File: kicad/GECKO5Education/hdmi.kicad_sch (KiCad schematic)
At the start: 20 parts, among them J2 HDMI_A, U3 PCA9306DQER, U6 LFE5U-85F-6BG381x

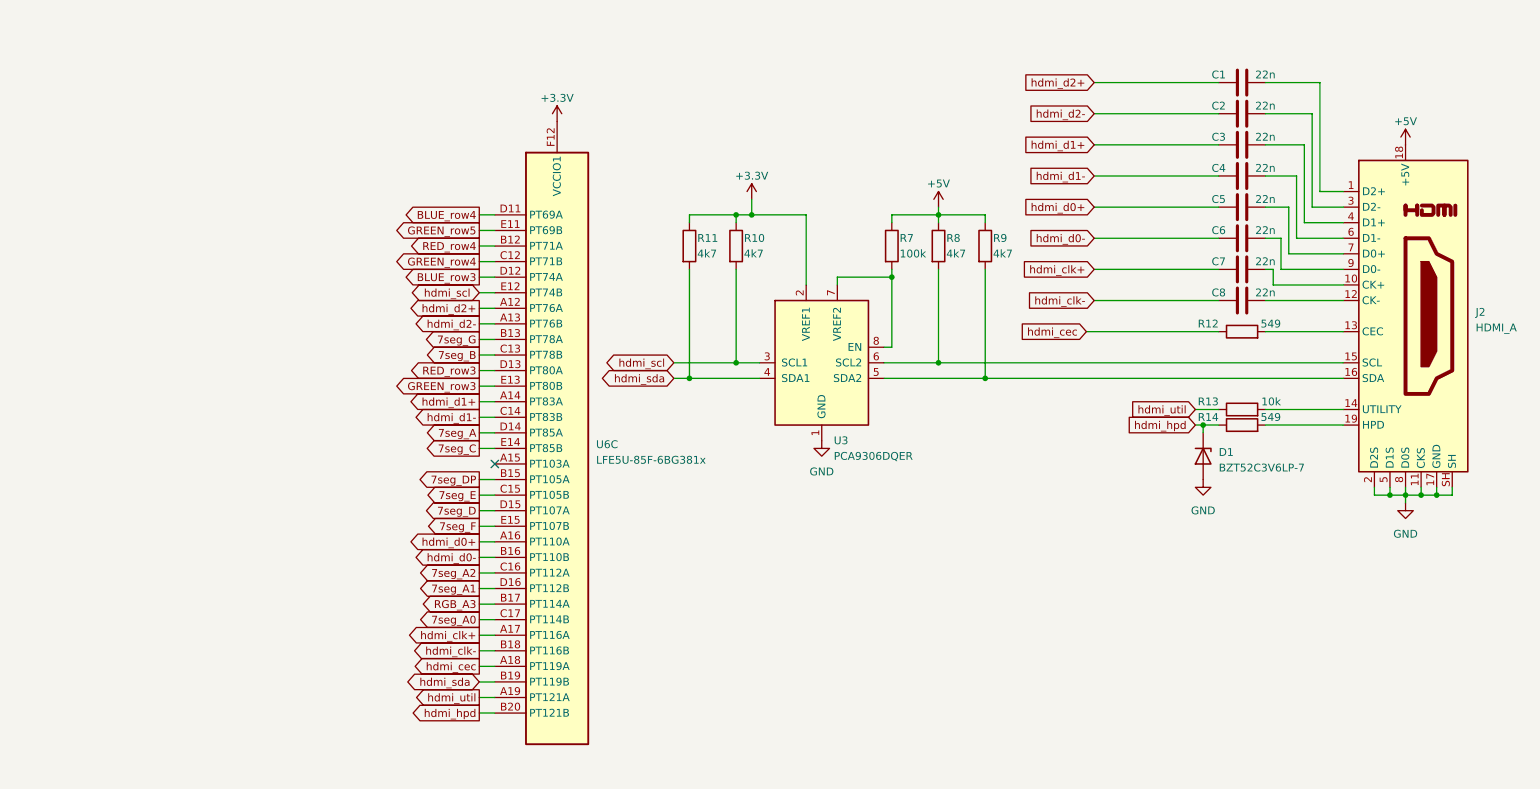
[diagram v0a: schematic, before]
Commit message: Made version V1.5
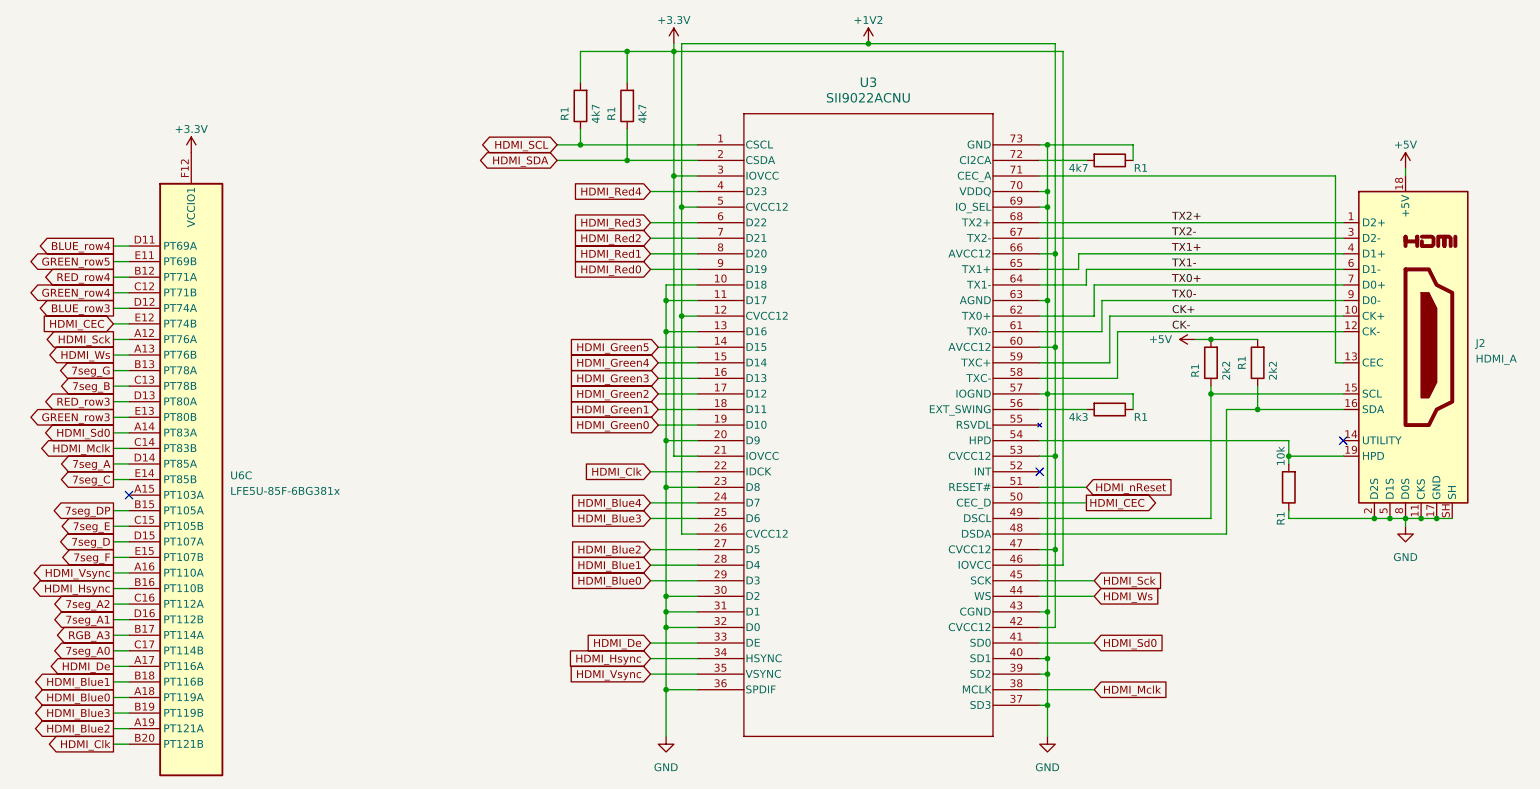
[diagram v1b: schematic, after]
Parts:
- removed C1, C2, C3, C4, C5, C6, C7, C8: 22n, Capacitor_SMD:C_0402_1005Metric, symbol Device:C
- removed D1: BZT52C3V6LP-7, Diode_SMD:D_0402_1005Metric, symbol Device:D_Zener
- removed R10, R11, R8, R9: 4k7, Resistor_SMD:R_0402_1005Metric, symbol Device:R
- removed R12, R14: 549, Resistor_SMD:R_0402_1005Metric, symbol Device:R
- removed R13: 10k, Resistor_SMD:R_0402_1005Metric, symbol Device:R
- removed R7: 100k, Resistor_SMD:R_0402_1005Metric, symbol Device:R
- removed U3: PCA9306DQER, Package_SON:X2SON-8_1.4x1mm_P0.35mm, symbol Interface:PCA9306
- added R1 (x3): 4k7, Resistor_SMD:R_0402_1005Metric, symbol Device:R
- added R1: 10k, Resistor_SMD:R_0402_1005Metric, symbol Device:R
- added R1: 4k3, Resistor_SMD:R_0402_1005Metric, symbol Device:R
- added R1 (x2): 2k2, Resistor_SMD:R_0402_1005Metric, symbol Device:R
- added U3: SII9022ACNU, gecko4education:QFN72_10X10_LAT-M, symbol gecko5education:SII9022ACNU
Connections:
- net +3.3V: now also R1.2, R1.2, U3.21 (IOVCC), U3.3 (IOVCC), U3.46 (IOVCC)
- net +5V: now also R1.2, R1.2
- net GND: now also R1.1, R1.1, R1.1, U3.10 (D18), U3.11 (D17), U3.13 (D16), U3.20 (D9), U3.23 (D8), U3.30 (D2), U3.31 (D1), U3.32 (D0), U3.36 (SPDIF), U3.37 (SD3), U3.39 (SD2), U3.40 (SD1), U3.43 (CGND), U3.57 (IOGND), U3.63 (AGND), U3.69 (IO_SEL), U3.70 (VDDQ), U3.73 (GND)
- net at J2.13 (CEC): now also U3.71 (CEC_A)
- net CK+: now reaches J2.10 (CK+)
- net CK+: now also U3.59 (TXC+)
- net CK-: now reaches J2.12 (CK-)
- net CK-: now also U3.58 (TXC-)
- net TX2+: now reaches J2.1 (D2+)
- net TX2+: now also U3.68 (TX2+)
- net TX1-: now reaches J2.6 (D1-)
- net TX1-: now also U3.64 (TX1-)
- net TX0+: now reaches J2.7 (D0+)
- net TX0+: now also U3.62 (TX0+)
- net TX1+: now reaches J2.4 (D1+)
- net TX1+: now also U3.65 (TX1+)
- net at J2.15 (SCL): now also R1.1, U3.49 (DSCL)
- net at J2.16 (SDA): now also R1.1, U3.48 (DSDA)
- net at J2.19 (HPD): now also R1.2, U3.54 (HPD)
- net TX2-: now reaches J2.3 (D2-)
- net TX2-: now also U3.67 (TX2-)
- net TX0-: now reaches J2.9 (D0-)
- net TX0-: now also U3.61 (TX0-)
- net hdmi_cec renamed HDMI_Blue0
- net HDMI_Blue0: now also U3.29 (D3)
- net hdmi_clk+ renamed HDMI_De
- net HDMI_De: now also U3.33 (DE)
- net hdmi_clk- renamed HDMI_Blue1
- net HDMI_Blue1: now also U3.28 (D4)
- net hdmi_d0+ renamed HDMI_Vsync
- net HDMI_Vsync: now also U3.35 (VSYNC)
- net hdmi_d0- renamed HDMI_Hsync
- net HDMI_Hsync: now also U3.34 (HSYNC)
- net hdmi_d1+ renamed HDMI_Sd0
- net HDMI_Sd0: now also U3.41 (SD0)
- net hdmi_d1- renamed HDMI_Mclk
- net HDMI_Mclk: now also U3.38 (MCLK)
- net hdmi_d2+ renamed HDMI_Sck
- net HDMI_Sck: now also U3.45 (SCK)
- net hdmi_d2- renamed HDMI_Ws
- net HDMI_Ws: now also U3.44 (WS)
- net hdmi_hpd renamed HDMI_Clk
- net HDMI_Clk: now also U3.22 (IDCK)
- net hdmi_scl renamed HDMI_CEC
- net HDMI_CEC: now also U3.50 (CEC_D)
- net hdmi_sda renamed HDMI_Blue3
- net HDMI_Blue3: now also U3.25 (D6)
- net hdmi_util renamed HDMI_Blue2
- net HDMI_Blue2: now also U3.27 (D5)
- new net: R1.2, U3.56 (EXT_SWING)
- new net: R1.2, U3.72 (CI2CA)
- new net +1V2: U3.12 (CVCC12), U3.26 (CVCC12), U3.42 (CVCC12), U3.47 (CVCC12), U3.5 (CVCC12), U3.53 (CVCC12), U3.60 (AVCC12), U3.66 (AVCC12)
- new net HDMI_Blue4: U3.24 (D7)
- new net HDMI_Green0: U3.19 (D10)
- new net HDMI_Green1: U3.18 (D11)
- new net HDMI_Green2: U3.17 (D12)
- new net HDMI_Green3: U3.16 (D13)
- new net HDMI_Green4: U3.15 (D14)
- new net HDMI_Green5: U3.14 (D15)
- new net HDMI_Red0: U3.9 (D19)
- new net HDMI_Red1: U3.8 (D20)
- new net HDMI_Red2: U3.7 (D21)
- new net HDMI_Red3: U3.6 (D22)
- new net HDMI_Red4: U3.4 (D23)
- new net HDMI_SCL: R1.1, U3.1 (CSCL)
- new net HDMI_SDA: R1.1, U3.2 (CSDA)
- new net HDMI_nReset: U3.51 (RESET#)
- no-connect marks 1 -> 3
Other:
- moved on the sheet: J2, U6C
